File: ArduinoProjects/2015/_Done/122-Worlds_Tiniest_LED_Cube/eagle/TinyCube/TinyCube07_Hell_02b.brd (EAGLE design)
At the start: 31.4 x 31.7 mm, 4 parts

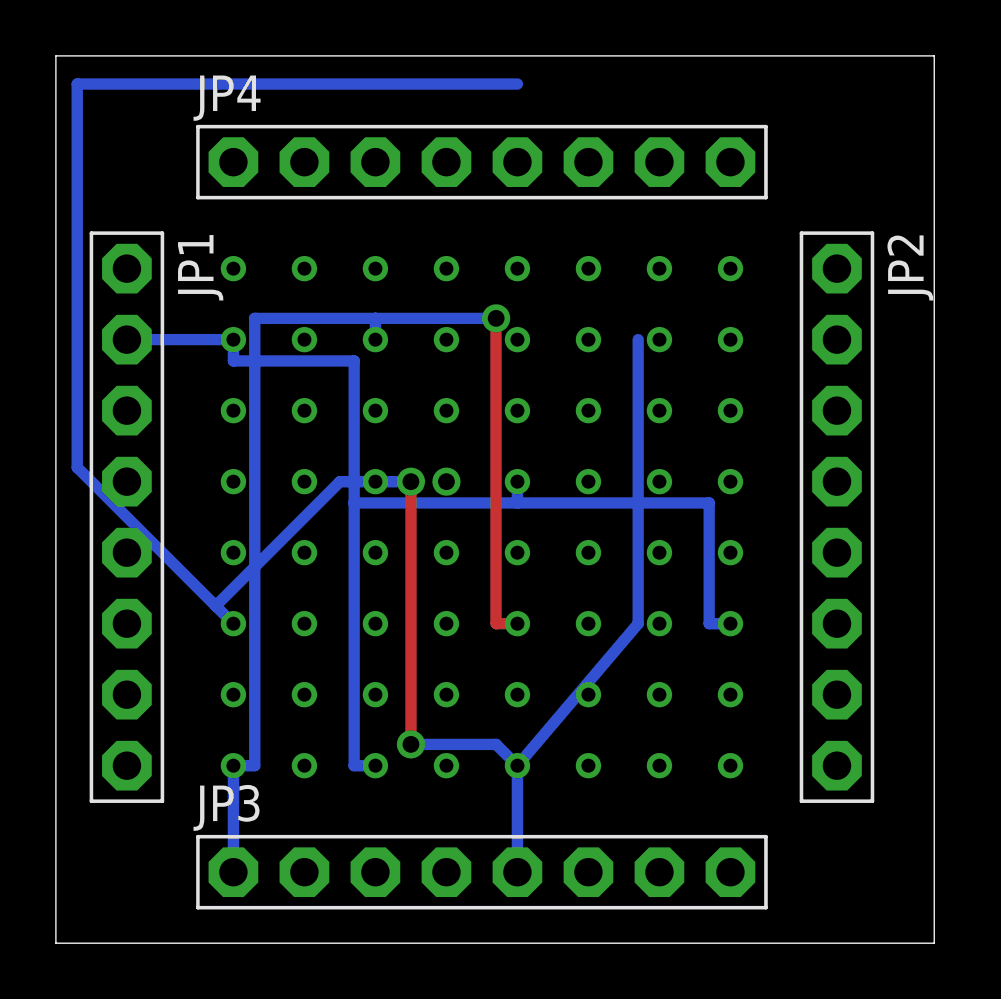
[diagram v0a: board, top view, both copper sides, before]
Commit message: sync
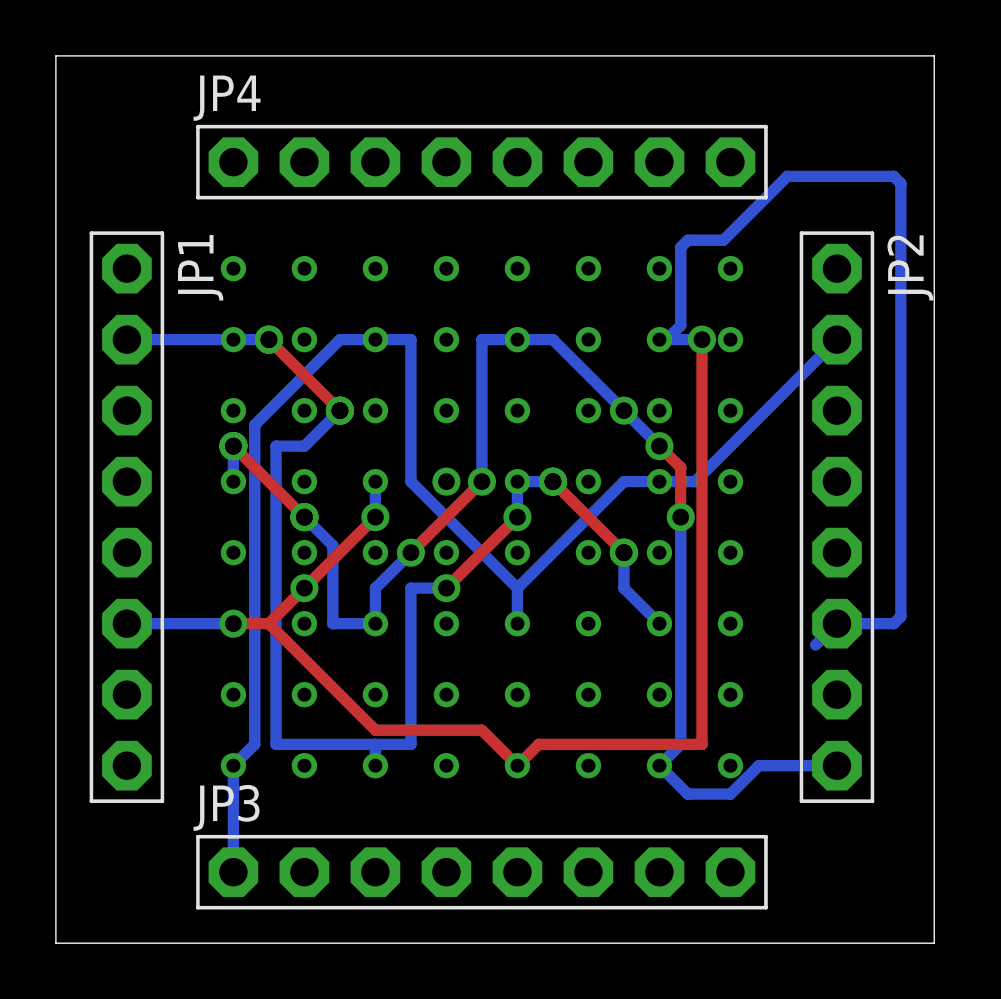
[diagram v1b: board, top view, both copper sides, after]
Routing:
- net N$77: track 80.4 -> 0.00 mm, vias 2 -> 0
- net N$8: track 0.00 -> 77.2 mm, vias 0 -> 3
- net N$10: track 0.00 -> 49.5 mm, vias 0 -> 7
- net N$1: track 42.7 -> 75.5 mm, vias 0 -> 6
- net N$73: track 41.7 -> 21.9 mm, vias 1 -> 0
